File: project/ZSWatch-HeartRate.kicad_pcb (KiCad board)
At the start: 2 copper layers, 27.5 x 18.2 mm, 19 parts, among them IC101 MAX32664, IC102 MAXM86161, X101 Mainboard, Y101 32kHz

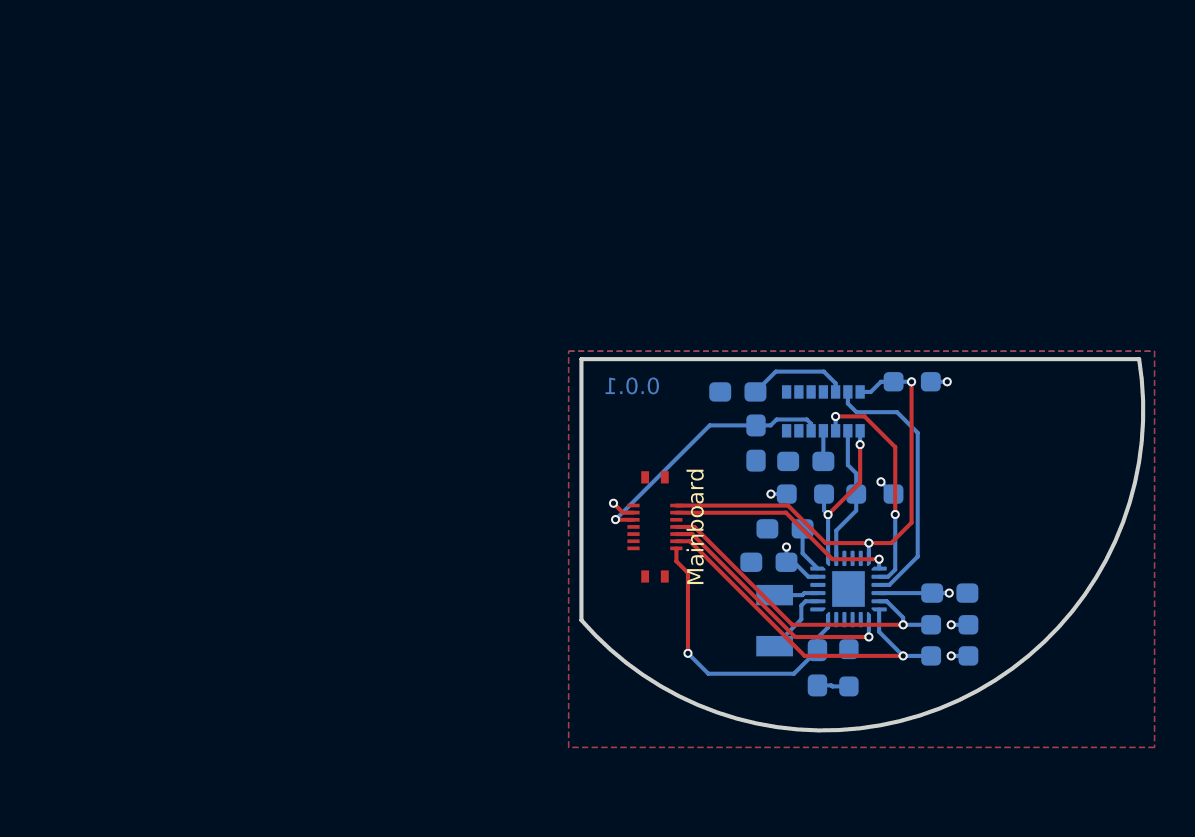
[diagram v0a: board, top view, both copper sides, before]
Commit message: First dev board version
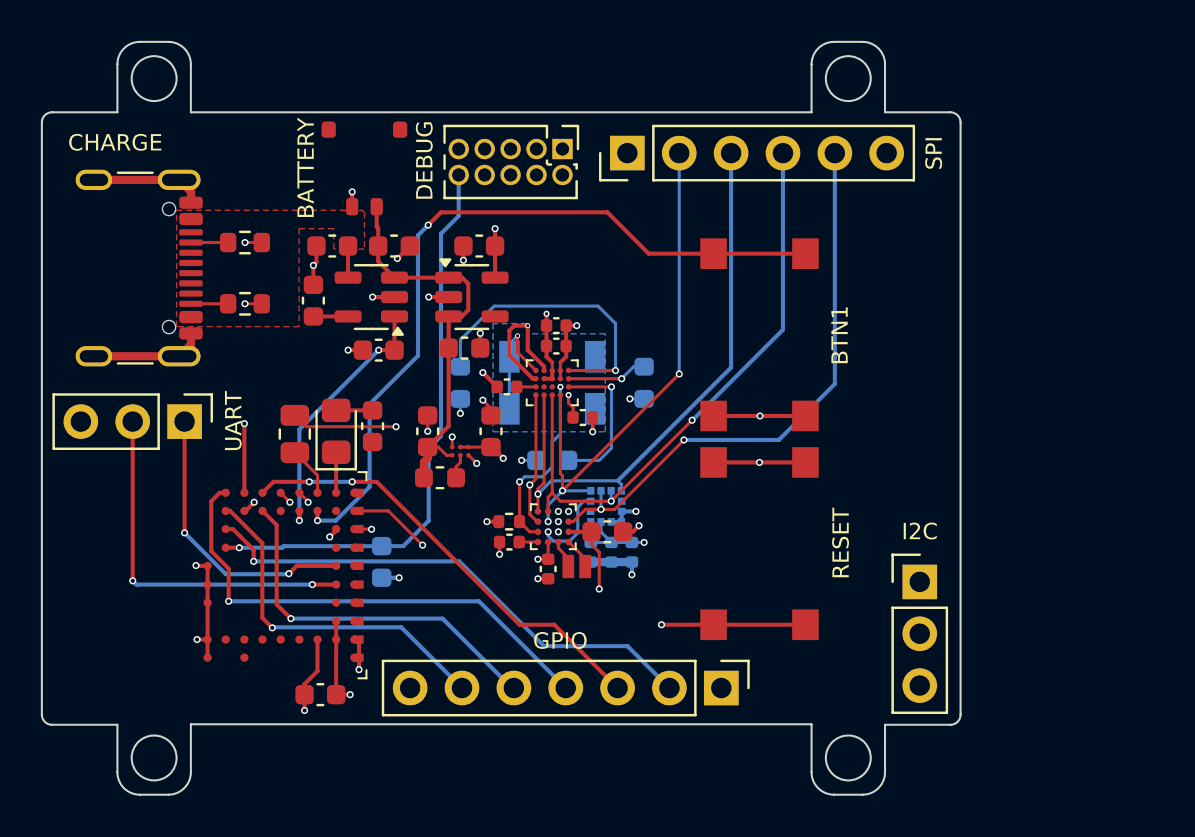
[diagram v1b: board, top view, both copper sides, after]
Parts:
- removed G*** (x2): LOGO, LOGO
- removed X101: Mainboard, Amphenol:101R014FB110
- added C108: 4u7, Capacitor_SMD:C_0603_1608Metric, F.Cu at (163.2, 103.4)
- added C109: 100n, Capacitor_SMD:C_0603_1608Metric, F.Cu at (154.8, 116.3)
- added C110: 1u, Capacitor_SMD:C_0603_1608Metric, F.Cu at (162.6, 94.3)
- added C111: 1u, Capacitor_SMD:C_0402_1005Metric, F.Cu at (166.0, 110.2)
- added C112: 1u, Capacitor_SMD:C_0402_1005Metric, F.Cu at (164.1, 108.8)
- added C113: 1u, Capacitor_SMD:C_0603_1608Metric, F.Cu at (161.9, 99.3)
- added C114: 100n, Capacitor_SMD:C_0402_1005Metric, B.Cu at (169.1, 109.3)
- added C115: 10u, Capacitor_SMD:C_0402_1005Metric, B.Cu at (170.1, 109.3)
- added C116: 100n, Capacitor_SMD:C_0402_1005Metric, B.Cu at (168.1, 109.3)
- added D102: D_Photo, Vishay:VEMD5080X01, B.Cu at (166.2, 101.0)
- added D104: RED, Diode_SMD:D_0603_1608Metric, B.Cu at (170.7, 101.0)
- added D105: IR, Diode_SMD:D_0603_1608Metric, B.Cu at (161.7, 101.0)
- added D106: GREEN, Diode_SMD:D_0603_1608Metric, B.Cu at (166.2, 104.8)
- added D107: STATUS, LED_SMD:LED_0805_2012Metric_Pad1.15x1.40mm_HandSolder, F.Cu at (155.6, 103.4)
- added IC103: MAX32664, Package_BGA_Kampi:WLP-16_2x2mm_P0.5mm, F.Cu at (166.2, 108.1)
- added IC104: TPS61240, Package_BGA_Kampi:DSBGA-6_0.886x1.288mm_2x3_P0.4mm, F.Cu at (161.7, 104.4)
- added IC105: MAX86141, Package_BGA_Kampi:THIN-WLP-20_2.228x1.967mm_P0.4mm, F.Cu at (166.2, 101.0)
- added IC106: MIC5365-1.8, Package_TO_SOT_SMD:SOT-23-5, F.Cu at (162.3, 96.8)
- added J101: SPI, Connector_PinHeader_2.54mm:PinHeader_1x06_P2.54mm_Vertical, F.Cu at (169.9, 89.8)
- added J102: GPIO, Connector_PinHeader_2.54mm:PinHeader_1x07_P2.54mm_Vertical, F.Cu at (174.5, 116.0)
- added J103: UART, Connector_PinHeader_2.54mm:PinHeader_1x03_P2.54mm_Vertical, F.Cu at (148.2, 103.0)
- added J104: I2C, Connector_PinHeader_2.54mm:PinHeader_1x03_P2.54mm_Vertical, F.Cu at (184.2, 110.8)
- added L101: 1u, Inductor_SMD:L_0603_1608Metric, F.Cu at (160.7, 105.7)
- added M101: BM15C, Fanstel:BM15C, F.Cu at (148.2, 110.5)
- added R107: 10k, Capacitor_SMD:C_0603_1608Metric, F.Cu at (157.7, 99.5)
- added R108: 10k, Capacitor_SMD:C_0603_1608Metric, B.Cu at (157.8, 109.8)
- added R109: 0R, Resistor_SMD:R_0805_2012Metric, F.Cu at (153.6, 103.6)
- added SW101: BTN1, Wuerth:WS-TASV-6x6, F.Cu at (176.3, 98.7)
- added SW102: RESET, Wuerth:WS-TASV-6x6, F.Cu at (176.3, 108.9)
- added X102: CHARGE, Connector_USB:USB_C_Receptacle_GCT_USB4105-xx-A_16P_TopMnt_Horizontal, F.Cu at (144.8, 95.4)
- added X103: BATTERY, Molex:78171-0002, F.Cu at (157.0, 90.5)
- added X104: DEBUG, Connector_PinHeader_1.27mm:PinHeader_2x05_P1.27mm_Vertical, F.Cu at (166.7, 89.6)
- C101: value 100n -> 4u7; footprint Capacitor_SMD:C_0603_1608Metric_Pad1.08x0.95mm_HandSolder -> Capacitor_SMD:C_0603_1608Metric; moved to F.Cu
- C102: value 1u -> 4u7; footprint Capacitor_SMD:C_0603_1608Metric_Pad1.08x0.95mm_HandSolder -> Capacitor_SMD:C_0603_1608Metric; moved to F.Cu
- C103: value 1u -> 100n; footprint Capacitor_SMD:C_0603_1608Metric_Pad1.08x0.95mm_HandSolder -> Capacitor_SMD:C_0402_1005Metric; moved to F.Cu
- C104: footprint Capacitor_SMD:C_0603_1608Metric_Pad1.08x0.95mm_HandSolder -> Capacitor_SMD:C_0402_1005Metric; moved to F.Cu
- C105: value 1u -> 22u; footprint Capacitor_SMD:C_0603_1608Metric_Pad1.08x0.95mm_HandSolder -> Capacitor_SMD:C_0402_1005Metric; moved to F.Cu
- C106: value 1u -> 10u; footprint Capacitor_SMD:C_0603_1608Metric_Pad1.08x0.95mm_HandSolder -> Capacitor_SMD:C_0402_1005Metric; moved to F.Cu
- C107: value 1u -> 2u2; footprint Capacitor_SMD:C_0603_1608Metric_Pad1.08x0.95mm_HandSolder -> Capacitor_SMD:C_0603_1608Metric; moved to F.Cu
- IC101: value MAX32664 -> LIS2DS12; footprint Package_DFN_QFN:QFN-24-1EP_3x3mm_P0.4mm_EP1.75x1.6mm -> Package_LGA:LGA-12_2x2mm_P0.5mm
- IC102: value MAXM86161 -> MCP73832-2-OT; footprint AnalogDevices:MAXM86161 -> Package_TO_SOT_SMD:SOT-23-5; moved to F.Cu
- R101: value 10R -> 10k; footprint Resistor_SMD:R_0603_1608Metric_Pad0.98x0.95mm_HandSolder -> Capacitor_SMD:C_0603_1608Metric; moved to F.Cu
- R102, R104: value 4k7 -> 5k1; footprint Resistor_SMD:R_0603_1608Metric_Pad0.98x0.95mm_HandSolder -> Resistor_SMD:R_0603_1608Metric; moved to F.Cu
- R103: footprint Resistor_SMD:R_0603_1608Metric_Pad0.98x0.95mm_HandSolder -> Resistor_SMD:R_0402_1005Metric; moved to F.Cu
- R105: value 4k7 -> 220R; footprint Resistor_SMD:R_0603_1608Metric_Pad0.98x0.95mm_HandSolder -> Capacitor_SMD:C_0603_1608Metric; moved to F.Cu
- R106: value 4k7 -> 10k; footprint Resistor_SMD:R_0603_1608Metric_Pad0.98x0.95mm_HandSolder -> Capacitor_SMD:C_0603_1608Metric; moved to F.Cu
- Y101: footprint Crystal:Crystal_SMD_3215-2Pin_3.2x1.5mm -> Crystal_Kampi:ECS_ECX-1210; moved to F.Cu
- moved R102 40.0 mm to (151.2, 94.2), turned to 0 degrees
- moved C101 31.5 mm to (155.4, 94.3), turned to 180 degrees
- moved R106 29.6 mm to (154.5, 97.0), turned to 90 degrees
- moved R104 29.0 mm to (151.2, 97.2), turned to 180 degrees
- moved R105 24.8 mm to (157.4, 103.2), turned to 90 degrees
- moved C102 24.0 mm to (158.4, 94.3), turned to 0 degrees
- moved IC102 22.8 mm to (157.3, 96.8), turned to 180 degrees
- moved C103 22.8 mm to (166.4, 99.2), turned to 180 degrees
- moved R103 22.2 mm to (164.1, 107.8), turned to 0 degrees
- moved C107 18.6 mm to (160.1, 103.4), turned to 90 degrees
- moved C104 15.3 mm to (164.0, 101.2)
- moved R101 13.6 mm to (168.9, 108.3), turned to 0 degrees
- moved IC101 12.5 mm to (168.8, 107.1), turned to -90 degrees
- moved C105 11.3 mm to (166.4, 98.2), turned to 180 degrees
- moved Y101 10.0 mm to (167.4, 110.0), turned to 180 degrees
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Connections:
- C101 pad 1: /~{RESET} -> Net-(IC102-V_{DD})
- C101 pad 2: Net-(C101-Pad2) -> GND
- C102 pad 1: +1V8 -> /V_{BAT}
- C104 pad 1: Net-(IC101-VCore) -> Net-(IC105-VREF)
- C105 pad 1: /V_LED -> +1V8
- C106 pad 1: Net-(IC102-VREF) -> /V_{LED}
- C107 pad 1: Net-(IC102-VLDO) -> /V_{BAT}
- IC101 pad 1: /MFIO -> Net-(IC101-SCL/SCLK)
- IC101 pad 10: GND -> +1V8
- IC101 pad 11: +1V8 -> unconnected-(IC101-INT2-Pad11)
- IC101 pad 12: Net-(IC101-VCore) -> /INT_{ACC}
- IC101 pad 2: (no net) -> Net-(IC101-CS)
- IC101 pad 3: (no net) -> Net-(IC101-SDO/ADDR0)
- IC101 pad 4: (no net) -> Net-(IC101-SDA/SDI/SDO)
- IC101 pad 5: (no net) -> unconnected-(IC101-NC-Pad5)
- IC101 pad 6: /~{RESET} -> GND
- IC101 pad 8: Net-(IC101-32KOUT) -> GND
- IC101 pad 9: Net-(IC101-32KIN) -> +1V8
- IC102 pad 1: Net-(IC101-SDA_Sensor) -> /CHARGE
- IC102 pad 2: Net-(IC101-SCL_Sensor) -> GND
- IC102 pad 3: Net-(IC101-LDO_EN) -> /V_{BAT}
- IC102 pad 4: Net-(IC102-VLDO) -> Net-(IC102-V_{DD})
- IC102 pad 5: /V_LED -> Net-(IC102-PROG)
- R101 pad 1: GND -> /~{RESET_{HR}}
- R101 pad 2: Net-(C101-Pad2) -> GND
- R102 pad 1: +1V8 -> Net-(X102-CC1)
- R102 pad 2: /SCL -> GND
- R103 pad 2: /SDA -> Net-(IC103-INT_{PPG})
- R104 pad 1: +1V8 -> GND
- R104 pad 2: Net-(IC101-SDA_Sensor) -> Net-(X102-CC2)
- R105 pad 1: +1V8 -> +BATT
- R105 pad 2: Net-(IC101-SCL_Sensor) -> Net-(D107-A)
- R106 pad 1: +1V8 -> Net-(IC102-PROG)
- R106 pad 2: /INT_HR -> GND
- Y101 pad 1: Net-(IC101-32KIN) -> Net-(IC103-32k_{OUT})
- Y101 pad 2: Net-(IC101-32KOUT) -> Net-(IC103-32k_{IN})
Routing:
- net GND: track 1.17 -> 60.5 mm, vias 1 -> 29
- net /~{RESET}: track 14.3 -> 57.3 mm, vias 1 -> 2
- net Net-(M101-P2.03): track 0.00 -> 37.3 mm, vias 0 -> 2
- net Net-(IC103-CS_{PPG}): track 0.00 -> 32.3 mm, vias 0 -> 1
- net Net-(IC101-SDO/ADDR0): track 0.00 -> 30.0 mm, vias 0 -> 2
- net Net-(IC101-SDA/SDI/SDO): track 0.00 -> 28.9 mm, vias 0 -> 1
- net Net-(IC101-CS): track 0.00 -> 28.1 mm, vias 0 -> 2
- net Net-(IC101-SCL/SCLK): track 0.00 -> 26.8 mm, vias 0 -> 3
- net /SWDIO: track 0.00 -> 26.1 mm, vias 0 -> 1
- net Net-(J102-Pin_2): track 0.00 -> 25.3 mm, vias 0 -> 1
- net Net-(J102-Pin_4): track 0.00 -> 24.4 mm, vias 0 -> 1
- net /SWDCLK: track 0.00 -> 24.2 mm, vias 0 -> 1
- net /INT_HR: track 23.1 -> 0.00 mm, vias 2 -> 0
- net Net-(J102-Pin_3): track 0.00 -> 21.8 mm, vias 0 -> 2
- net /V_{BAT}: track 0.00 -> 19.7 mm
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- added copper zone on In1.Cu, net (none)
- added copper zone on In2.Cu, net +1V8
- added copper zone on In2.Cu, net /V_{LED}
- added copper zone on In1.Cu, net GND
- added copper zone on F.Cu, net Net-(IC102-V_{DD})
- removed copper zone on F.Cu, net +1V8
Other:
- board size 27.5 x 18.2 mm -> 45 x 36.9 mm
- copper layers 2 -> 4
- board text removed: "0.0.${REVISION}"
